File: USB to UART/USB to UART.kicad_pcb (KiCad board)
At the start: 2 copper layers, 70 x 48.5 mm, 19 parts, among them J1 USB_C_Receptacle_USB2.0_16P, J2 Conn_01x05_Pin, U1 CP2102N-Axx-xQFN28

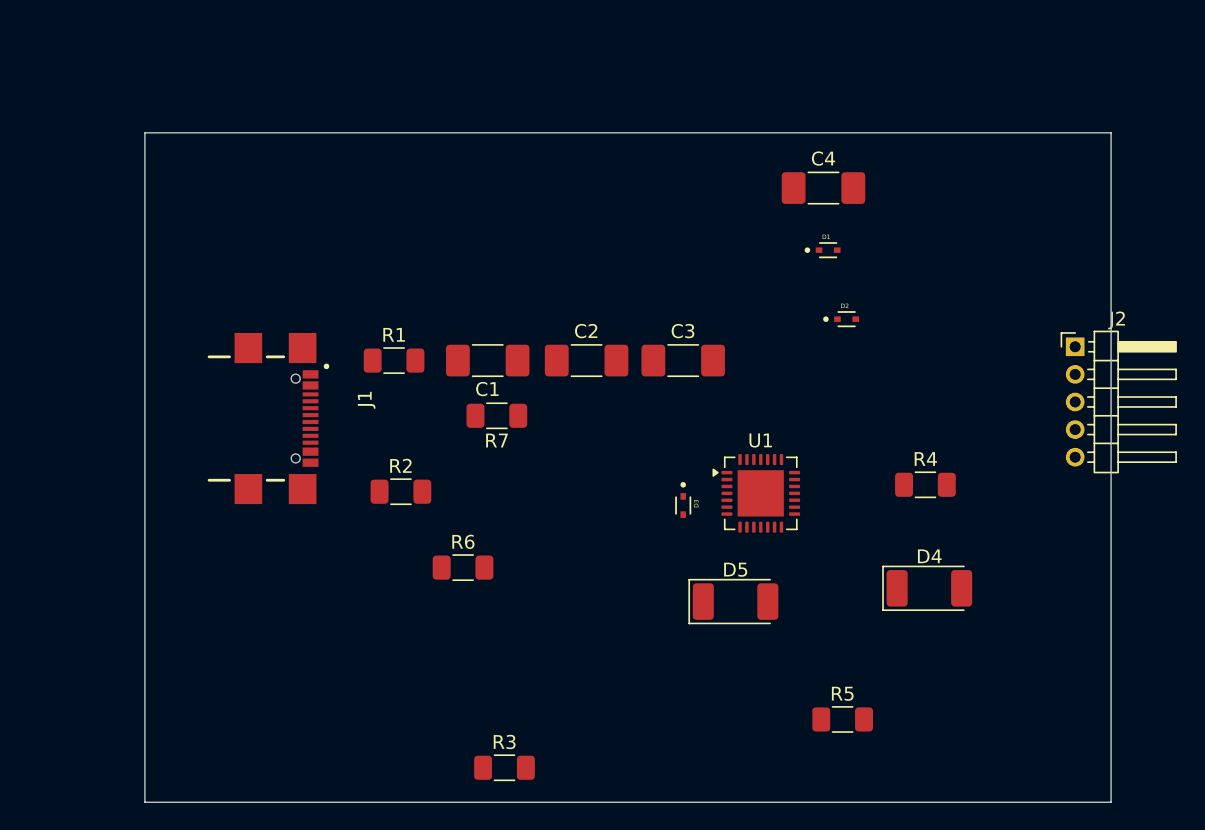
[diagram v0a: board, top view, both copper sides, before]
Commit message: screenshot added
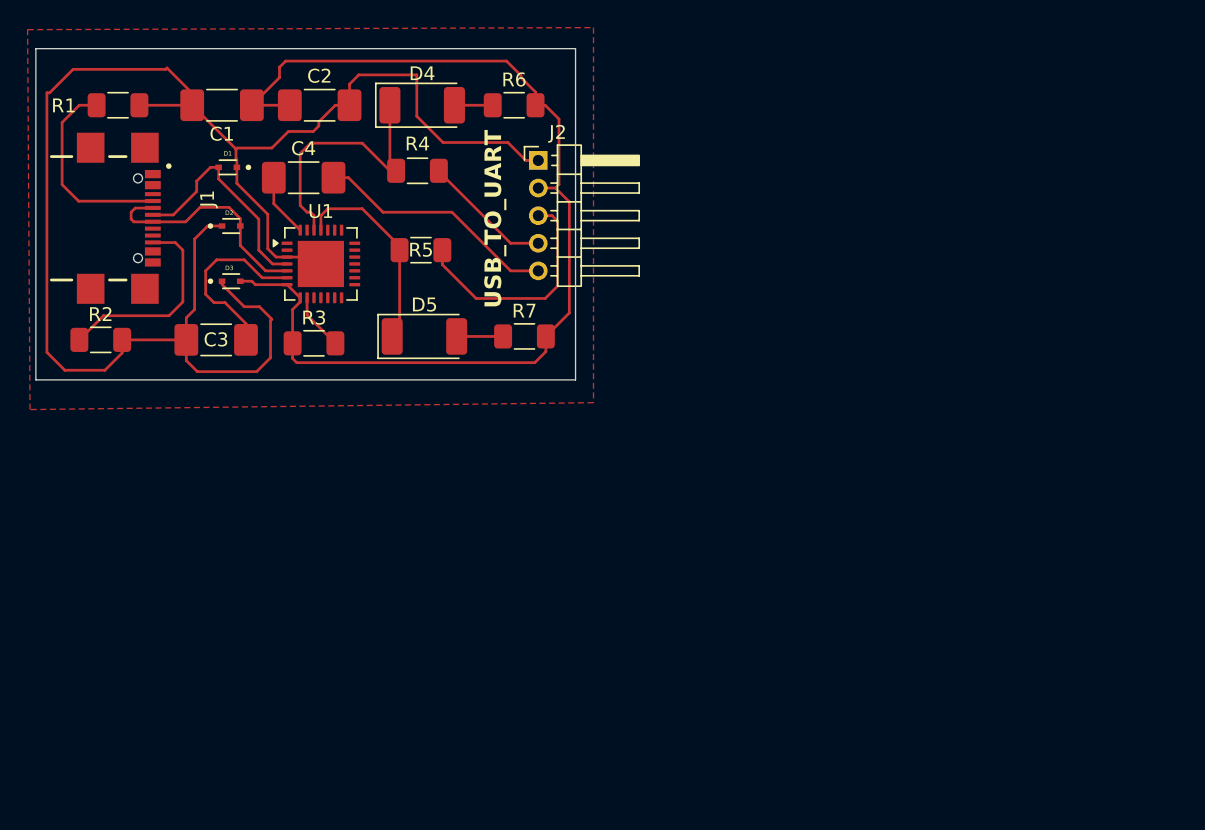
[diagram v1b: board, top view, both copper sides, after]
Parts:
- moved D4 50.8 mm to (75.1, 43.0)
- moved R5 45.7 mm to (75.0, 53.5)
- moved D2 45.1 mm to (61.2, 51.8)
- moved D1 43.9 mm to (61.0, 47.5), turned to 180 degrees
- moved R4 43.3 mm to (74.8, 47.8)
- moved J2 41.2 mm to (83.5, 47.0)
- moved C4 37.7 mm to (66.5, 48.2)
- moved D3 36.6 mm to (61.2, 55.8), turned to 0 degrees
- moved U1 35.9 mm to (67.8, 54.5)
- moved C3 33.9 mm to (60.2, 60.0)
- moved R3 33.7 mm to (67.2, 60.2)
- moved R6 33.7 mm to (81.8, 43.0)
- moved D5 29.6 mm to (75.2, 59.8)
- moved R1 27.2 mm to (53.0, 43.0)
- moved C2 26.8 mm to (67.7, 43.0)
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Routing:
- net GND: track 0.00 -> 120.1 mm
- net /vbus: track 0.00 -> 76.7 mm
- net Net-(D4-K): track 0.00 -> 19.1 mm
- net /RST: track 0.00 -> 17.6 mm
- net /-D: track 0.00 -> 17.4 mm
- net /RX: track 0.00 -> 17.1 mm
- net /+D: track 0.00 -> 16.2 mm
- net Net-(D5-K): track 0.00 -> 14.8 mm
- net Net-(J1-CC2): track 0.00 -> 14.7 mm
- net Net-(J1-CC1): track 0.00 -> 14.7 mm
- net Net-(U1-VDD): track 0.00 -> 13.5 mm
- net /TX: track 0.00 -> 9.40 mm
- net Net-(U1-~{DTR}): track 0.00 -> 4.59 mm
- net Net-(U1-~{RST}): track 0.00 -> 4.15 mm
- net Net-(D5-A): track 0.00 -> 3.36 mm
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- added copper zone on F.Cu, net GND
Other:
- board size 70 x 48.5 mm -> 39.1 x 24 mm
- board text added: "USB_TO_UART"
